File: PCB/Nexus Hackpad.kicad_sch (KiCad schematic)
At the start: 30 parts, among them SW1 SW_Push, SW10 RotaryEncoder_Switch, SW2 SW_Push, SW3 SW_Push, SW4 SW_Push, SW5 SW_Push, SW6 SW_Push, SW7 SW_Push, SW8 SW_Push, SW9 SW_Push, U1 MOUDLE-SEEEDUINO-XIAO, U2 ER_OLEDM0.91_1x-I2C

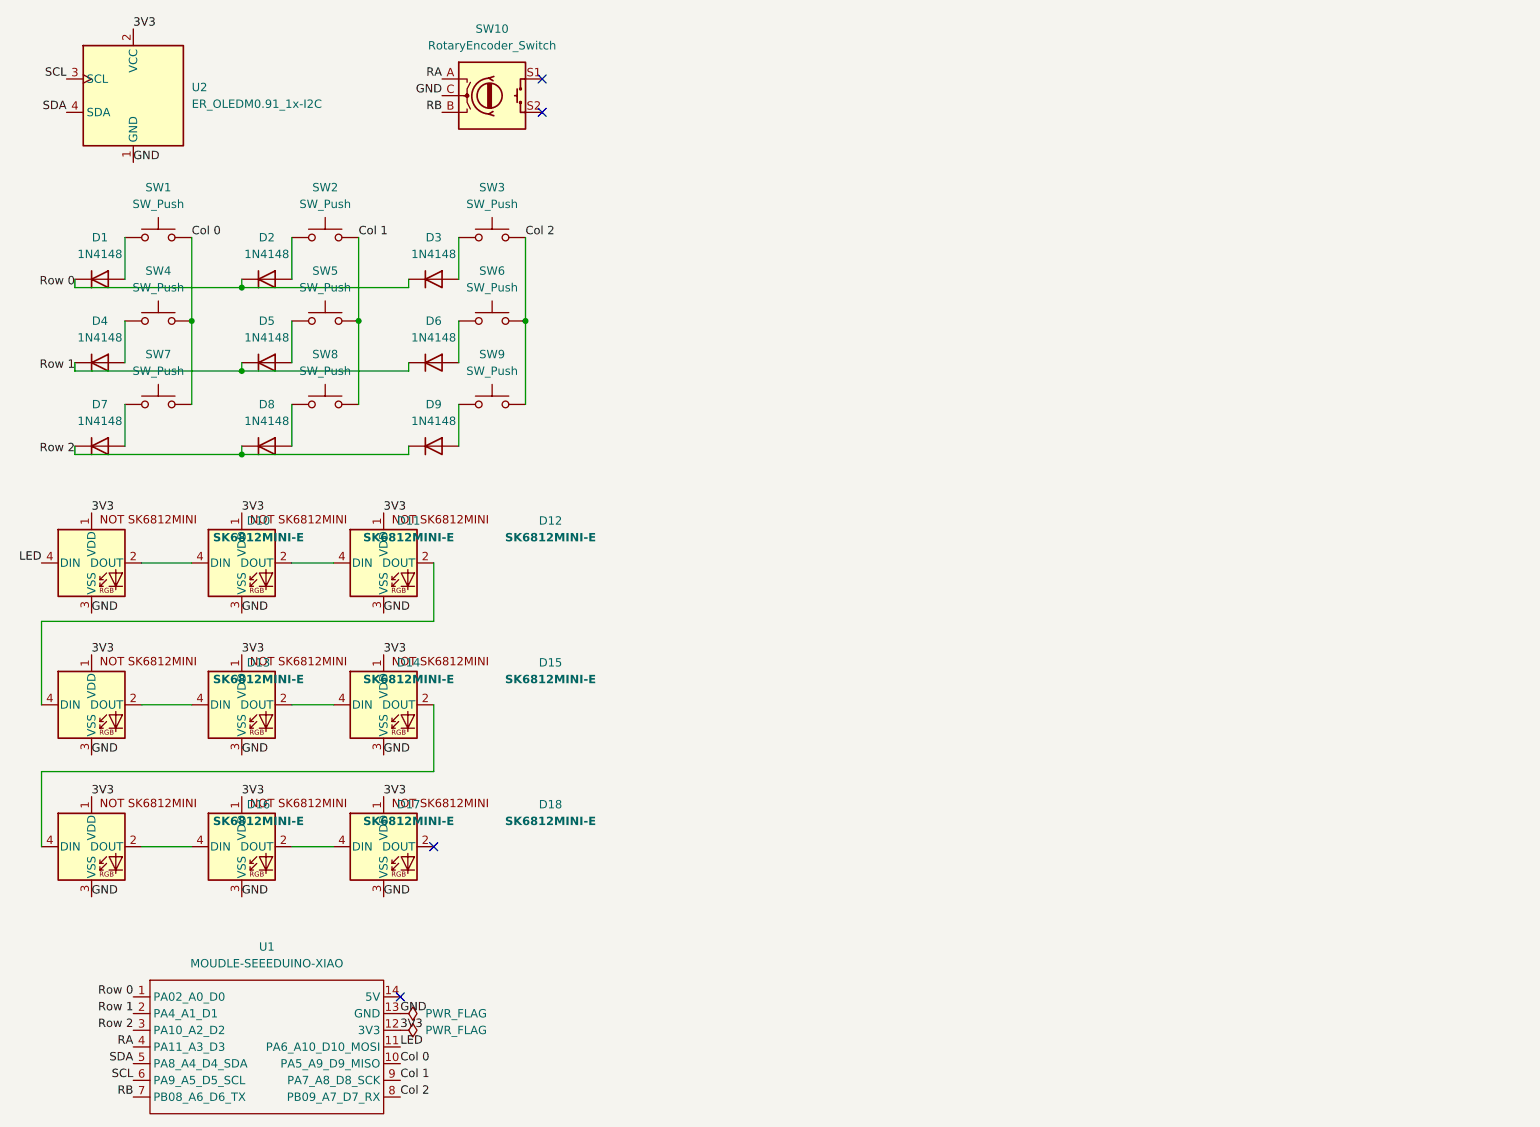
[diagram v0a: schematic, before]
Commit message: Merge branches 'main' and 'main' of https://github.com/ttayG-sr/Nexus-Hackpad
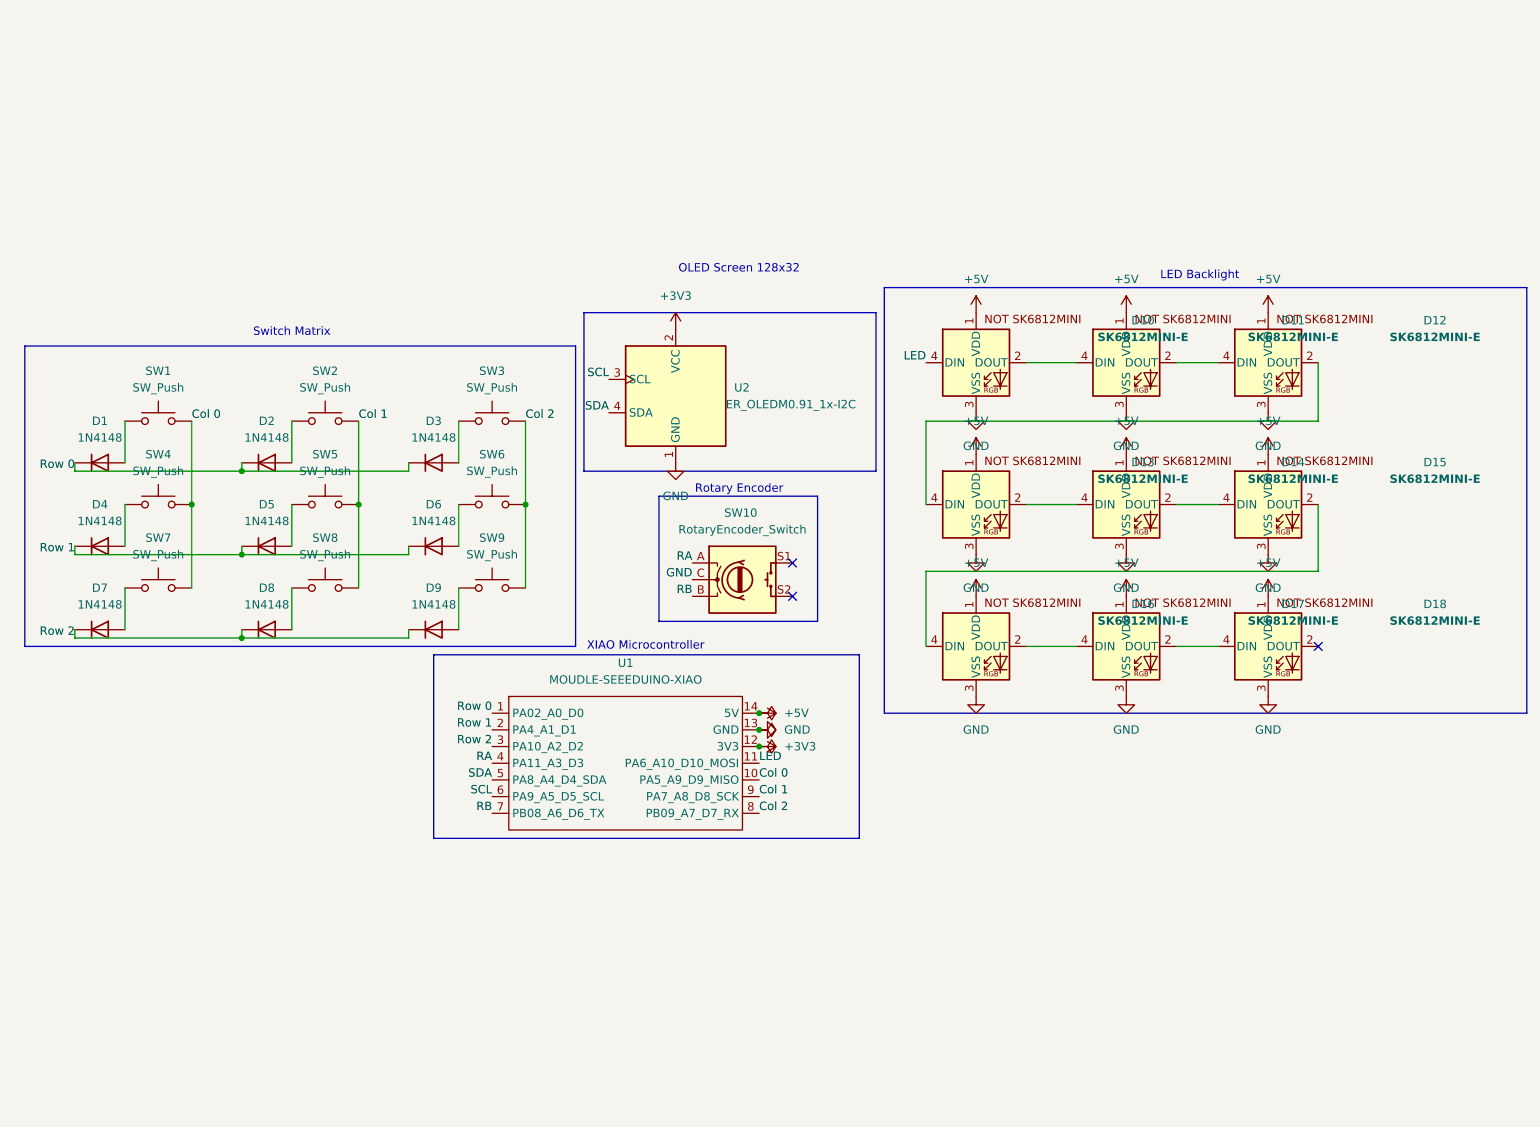
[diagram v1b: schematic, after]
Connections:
- net +5V: now reaches U1.14 (5V)
- net +5V: now also D10.1 (VDD), D11.1 (VDD), D12.1 (VDD), D13.1 (VDD), D14.1 (VDD), D15.1 (VDD), D16.1 (VDD), D17.1 (VDD), D18.1 (VDD)
- removed net 3V3: D10.1 (VDD), D11.1 (VDD), D12.1 (VDD), D13.1 (VDD), D14.1 (VDD), D15.1 (VDD), D16.1 (VDD), D17.1 (VDD), D18.1 (VDD), U1.12 (3V3), U2.2 (VCC)
- new net +3V3: U1.12 (3V3), U2.2 (VCC)
- no-connect marks 4 -> 3
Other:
- note added: "LED Backlight"
- note added: "OLED Screen 128x32"
- note added: "Rotary Encoder"
- note added: "Switch Matrix"
- note added: "XIAO Microcontroller"
- moved on the sheet: D1, D10, D11, D12, D13, D14, D15, D16, D17, D18, D2, D3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
